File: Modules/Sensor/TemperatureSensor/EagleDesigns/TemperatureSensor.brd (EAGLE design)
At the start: 100 x 80 mm, 7 parts, among them U1 TINY85-20-DIP

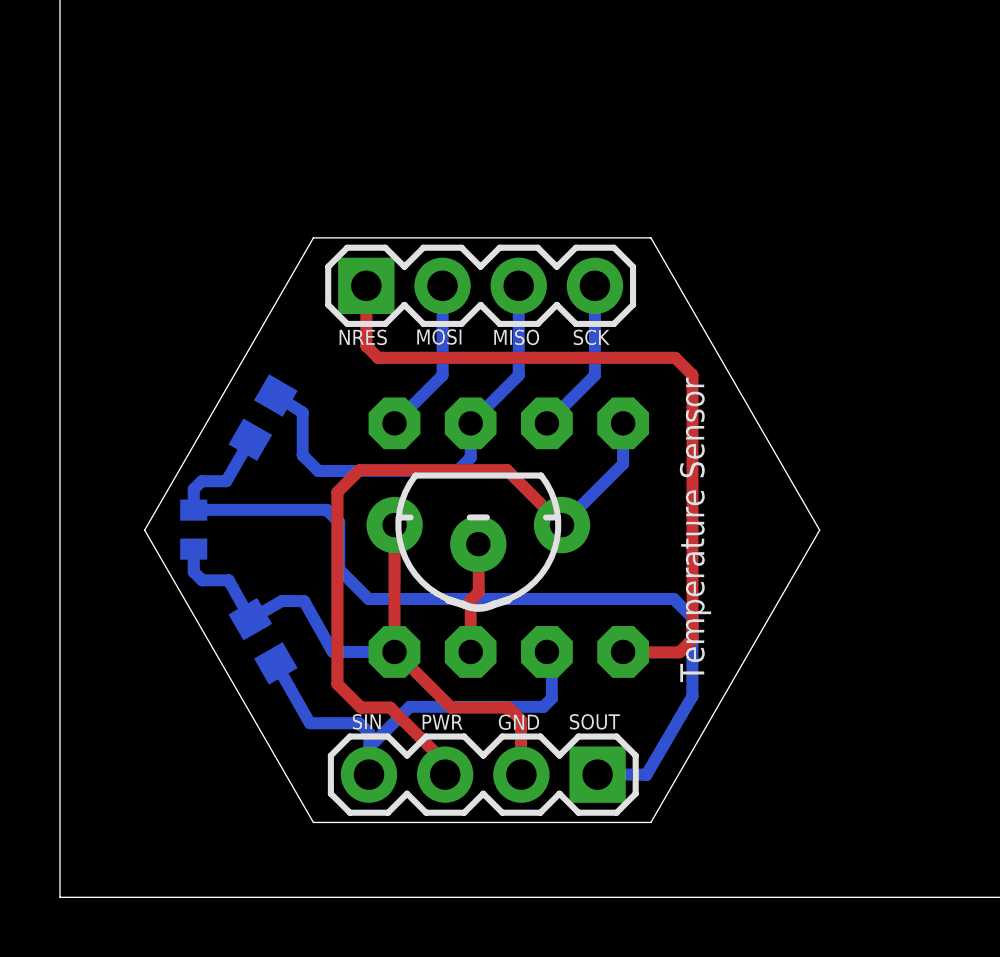
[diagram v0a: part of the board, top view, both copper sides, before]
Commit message: re-organized files after Merge
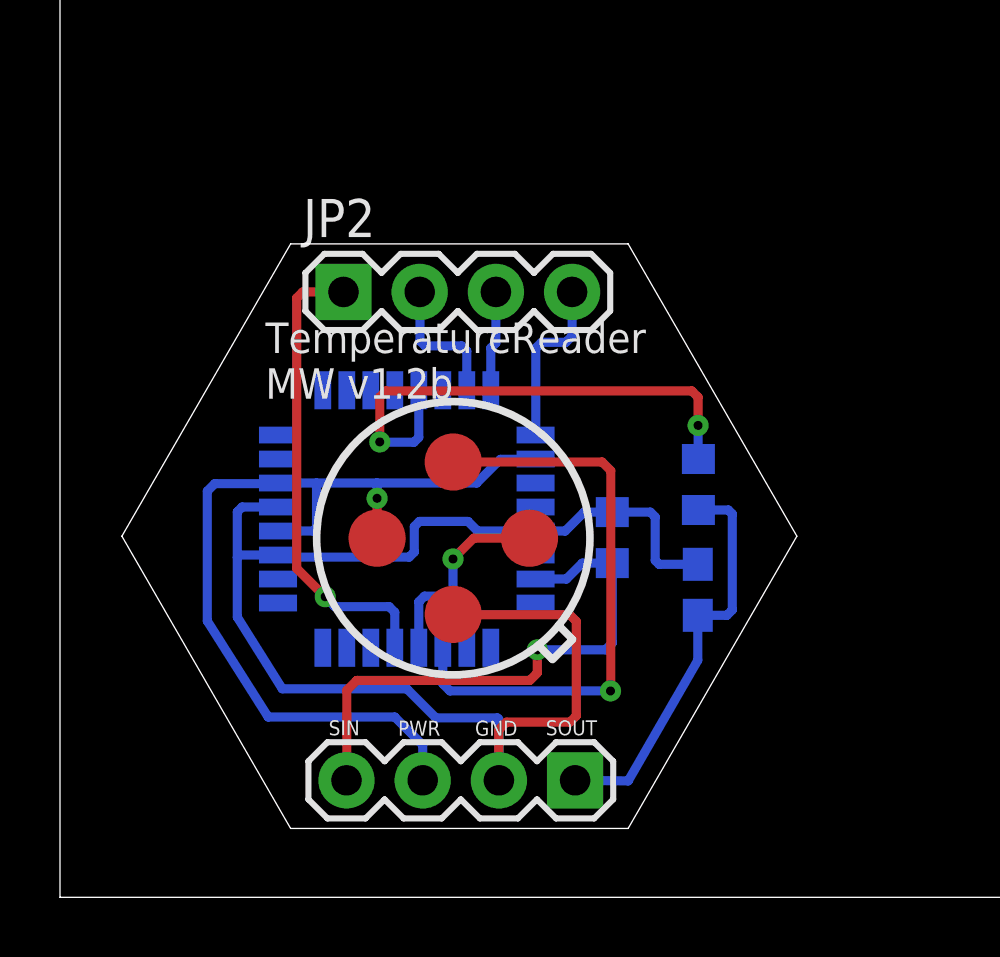
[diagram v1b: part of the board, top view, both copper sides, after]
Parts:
- removed C1: 0.22uF, adafruit:C0402
- removed R2: 4.7K, adafruit:R0603
- added C3: 0.22uF, adafruit:C0603
- added R4: 4.7K, adafruit:R0603
- U1: value TINY85-20-DIP -> MLX90614; device SparkFun-DigitalIC:DIP08 -> MakerWear:TO-39
- U2: value (none) -> ATMEGA328P_TQFP; device SparkFun-Sensors:TO-92 -> SparkFun-DigitalIC:TQFP32-08
- moved R1 12.1 mm to (18.4, 12.0), turned to 270 degrees
- moved U2 2.39 mm to (11.6, 12.6), flipped to the bottom
- moved U1 1.85 mm to (13.1, 12.0), flipped to the top
- moved JP2 0.79 mm to (9.45, 20.2)
- moved JP1 0.77 mm to (17.2, 3.90)
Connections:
- removed net NRES: JP2.1, U1.1
- removed net OUT(MISO): JP2.3, R2.2, U1.6
- removed net SENSOR: U1.3, U2.2
- new net MISO: JP2.3, U2.16
- new net OUT: R4.2, U2.13
- new net RESET: JP2.1, U2.29
- new net SCL: U1.SCL, U2.28
- new net SDA: U1.PWM, U2.27
- net 1X3SIN: now also U2.23; no longer U1.2
- net 1X3SOUT: now also C3.1, R4.1; no longer C1.2, R2.1
- net GND: now also C3.2, U1.VSS, U2.21, U2.5; no longer C1.1, U1.4
- net MOSI: now also U2.15; no longer U1.5
- net SCK: now also U2.17; no longer U1.7
- net VCC: now also U1.VDD, U2.18, U2.4, U2.6; no longer U1.8, U2.1
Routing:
- net GND: track 20.7 -> 47.6 mm
- net NRES: track 24.6 -> 0.00 mm
- net SDA: track 0.00 -> 19.6 mm, vias 0 -> 1
- net OUT: track 0.00 -> 17.3 mm, vias 0 -> 2
- net 1X3SOUT: track 29.8 -> 13.5 mm
- net RESET: track 0.00 -> 15.7 mm, vias 0 -> 1
- net OUT(MISO): track 14.9 -> 0.00 mm
- net SCL: track 0.00 -> 6.74 mm, vias 0 -> 1
- net VCC: track 24.3 -> 30.9 mm, vias 0 -> 1
- net SENSOR: track 3.71 -> 0.00 mm
- net MISO: track 0.00 -> 3.35 mm
- net 1X3SIN: track 15.1 -> 18.4 mm, vias 0 -> 1
- net MOSI: track 5.25 -> 4.64 mm
- net SCK: track 5.25 -> 5.75 mm
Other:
- outline, holes or cut-outs redrawn
- board text added: "TemperatureReader MW v1.2b"
- board text removed: "MISO"
- board text removed: "MOSI"
- board text removed: "MW-V3"
- board text removed: "NRES"
- board text removed: "SCK"
- board text removed: "Temperature Sensor"
